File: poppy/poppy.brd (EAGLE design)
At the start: 100 x 80 mm, 16 parts, among them Q1 10MHz, U1 ATUSB, U2 MBI5039

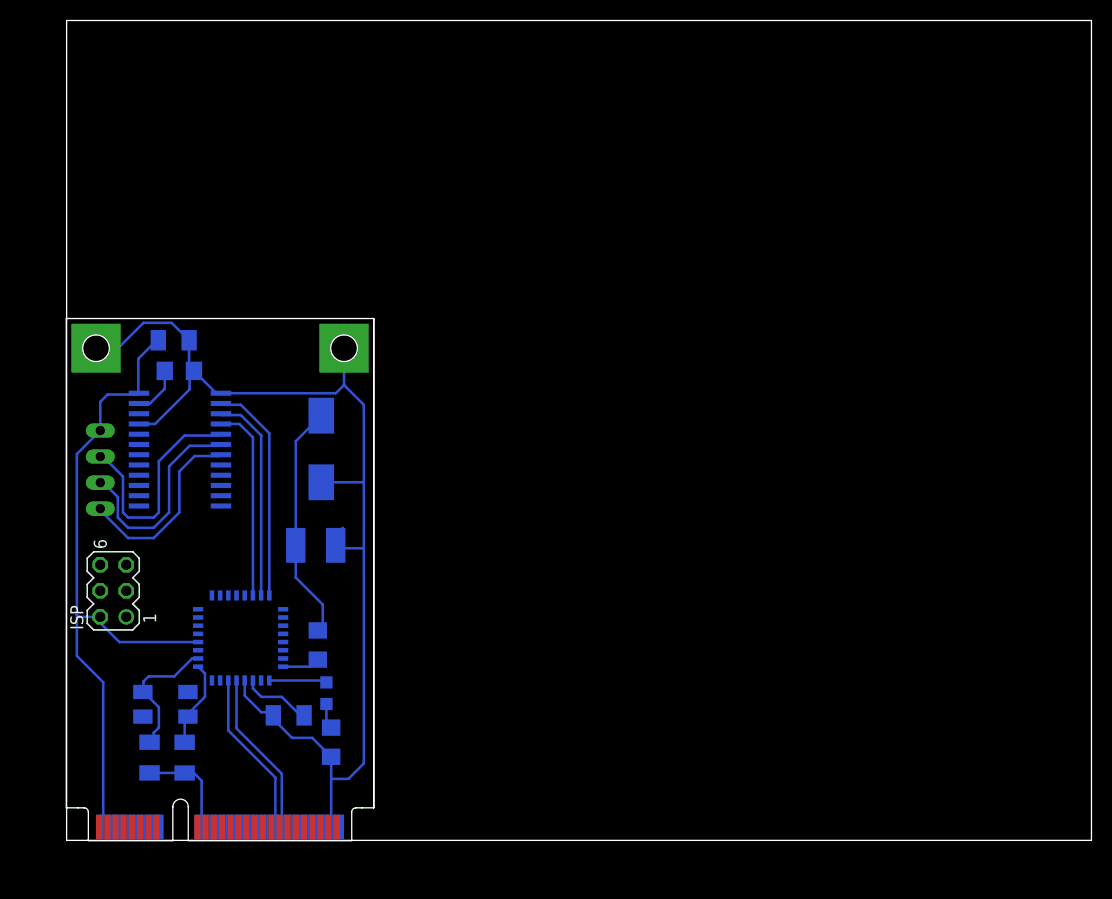
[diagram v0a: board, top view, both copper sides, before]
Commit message: Ready to etch!
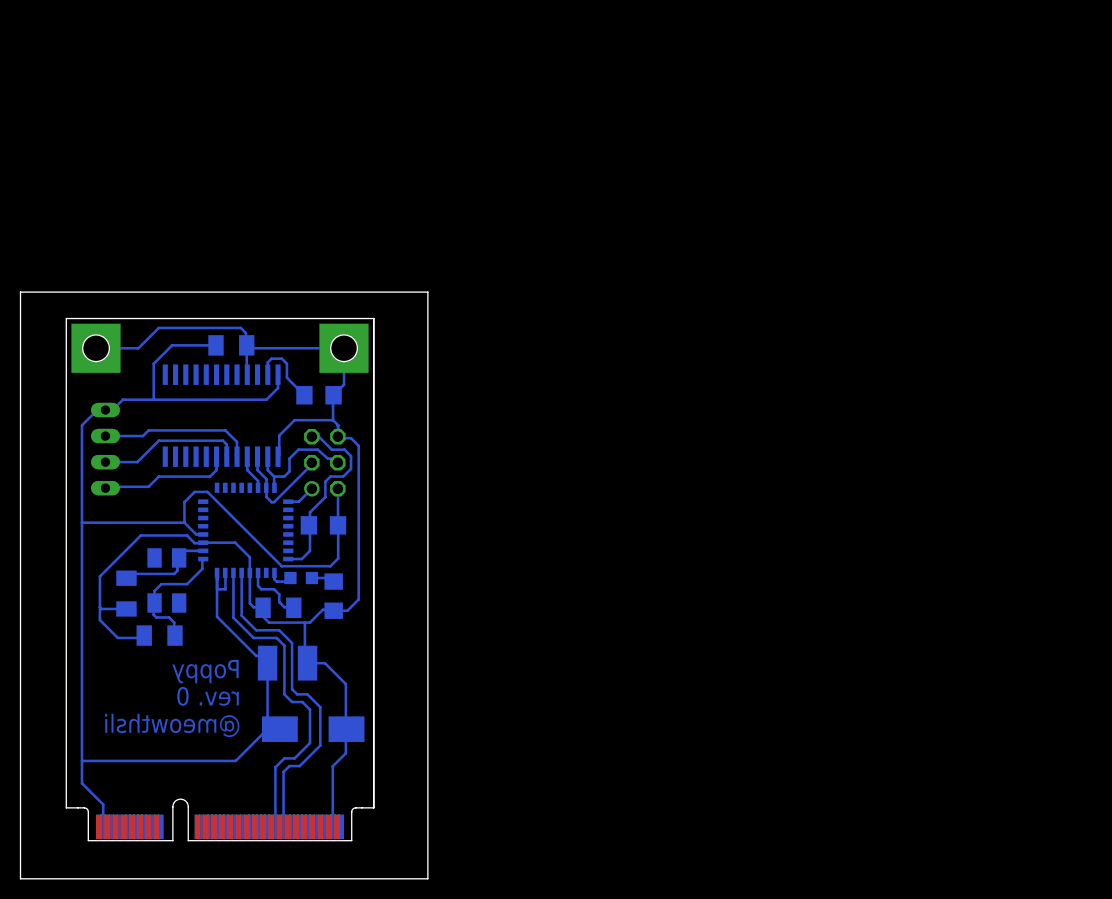
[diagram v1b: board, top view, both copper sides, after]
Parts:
- moved C2 27.4 mm to (24.1, 10.8), turned to 0 degrees
- moved ISP 24.1 mm to (25.2, 36.9), flipped to the bottom
- moved C4 16.2 mm to (5.84, 24.1)
- moved R2 14.3 mm to (26.1, 23.8)
- moved R3 13.8 mm to (24.6, 43.4)
- moved C3 12.2 mm to (9.07, 20.0), turned to 0 degrees
- moved Q1 12.1 mm to (9.78, 25.4), turned to 90 degrees
- moved C1 11.8 mm to (21.6, 17.3)
- moved R1 11.7 mm to (25.1, 30.7), turned to 180 degrees
- moved LED1 11.5 mm to (22.9, 25.6), turned to 90 degrees
- moved C5 10.5 mm to (20.7, 22.7)
- moved U1 10.5 mm to (17.5, 30.2)
- moved C6 5.65 mm to (16.1, 48.3)
- moved U2 5.36 mm to (15.2, 41.5), turned to 0 degrees
- moved LED2 2.06 mm to (3.79, 38.2)
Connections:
- removed net GND18: C3.2, C4.2, EDGE.18
- net GND: now also C3.2, C4.2
- net MISO: now also ISP.1; no longer ISP.5
- net MOSI/DATA: now also ISP.4; no longer ISP.1
- net RESET: now also ISP.5; no longer ISP.3
- net SCK: now also ISP.3; no longer ISP.4
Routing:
- net VCC: track 90.3 -> 156.1 mm
- net GND: track 112.9 -> 138.1 mm
- net D+: track 16.2 -> 31.9 mm
- net LATCH: track 19.1 -> 3.47 mm
- net D-: track 16.2 -> 31.8 mm
- net RESET: track 3.66 -> 18.9 mm
- net MOSI/DATA: track 21.7 -> 11.8 mm
- net GND18: track 9.90 -> 0.00 mm
- net SCK: track 20.4 -> 10.7 mm
- net N$3: track 22.6 -> 15.1 mm
- net N$5: track 20.8 -> 14.2 mm
- net N$6: track 18.8 -> 12.9 mm
- net XTAL1: track 8.47 -> 12.5 mm
- net XTAL2: track 13.3 -> 9.99 mm
- net MISO: track 0.00 -> 2.82 mm
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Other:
- board size 100 x 80 mm -> 39.8 x 57.2 mm
- board text added: "Poppy rev. 0 @meowthsli"
